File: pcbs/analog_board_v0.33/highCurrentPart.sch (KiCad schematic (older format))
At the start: 23 parts, among them J6 CONN_01X02, J7 CONN_01X02, J8 CONN_01X02, J9 CONN_01X02, Q1 MMBT3904, U3 LM358, U4 ICL7660S, U5 ICL7660S

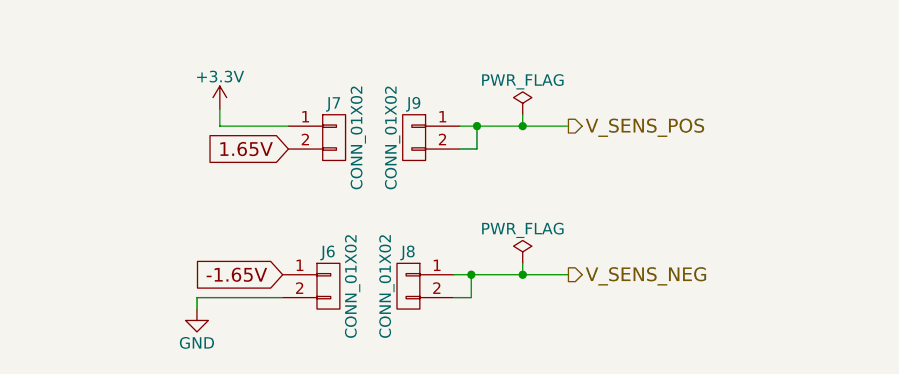
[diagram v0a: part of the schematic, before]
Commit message: Finished new BOM.
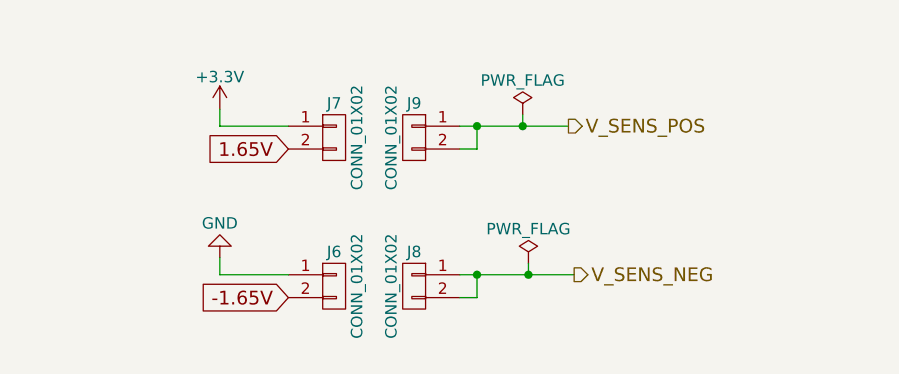
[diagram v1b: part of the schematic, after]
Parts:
- R10: Farnell 1632456 -> 9237364
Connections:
- net -1.65V: now also J6.2 (P2); no longer J6.1 (P1)
- net GND: now also J6.1 (P1); no longer J6.2 (P2)
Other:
- moved on the sheet: J6, J8
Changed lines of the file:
@@
 F 2 "Resistors_SMD:R_0805" V 1055 4025 50  0001 C CNN
 F 3 "" H 1125 4025 50  0000 C CNN
-F 4 "1632456" V 1125 4025 60  0001 C CNN "Farnell"
+F 4 "9237364" V 1125 4025 60  0001 C CNN "Farnell"
 	1    1125 4025
 	1    0    0    -1
@@
 	1    0    0    -1
 $EndComp
-Wire Wire Line
-	3575 5950 3875 5950
-Wire Wire Line
-	3575 5875 3575 5950
 Text HLabel 5100 5950 2    60   Output ~ 0
 V_SENS_POS
@@
 L CONN_01X02 J6
 U 1 1 5993FBA5
-P 4050 6650
-F 0 "J6" H 4050 6800 50  0000 C CNN
-F 1 "CONN_01X02" V 4150 6650 50  0000 C CNN
-F 2 "Samtec Connectors:Samtec-PHT-1-2-01-L-S" H 4050 6650 50  0001 C CNN
-F 3 "" H 4050 6650 50  0001 C CNN
-	1    4050 6650
+P 4075 6650
+F 0 "J6" H 4075 6800 50  0000 C CNN
+F 1 "CONN_01X02" V 4175 6650 50  0000 C CNN
+F 2 "Samtec Connectors:Samtec-PHT-1-2-01-L-S" H 4075 6650 50  0001 C CNN
+F 3 "" H 4075 6650 50  0001 C CNN
+	1    4075 6650
 	1    0    0    -1
 $EndComp
@@
 L CONN_01X02 J8
 U 1 1 5993FBAB
-P 4400 6650
-F 0 "J8" H 4400 6800 50  0000 C CNN
-F 1 "CONN_01X02" V 4500 6650 50  0000 C CNN
-F 2 "Samtec Connectors:Samtec-PHT-1-2-01-L-S" H 4400 6650 50  0001 C CNN
-F 3 "" H 4400 6650 50  0001 C CNN
-	1    4400 6650
+P 4425 6650
+F 0 "J8" H 4425 6800 50  0000 C CNN
+F 1 "CONN_01X02" V 4525 6650 50  0000 C CNN
+F 2 "Samtec Connectors:Samtec-PHT-1-2-01-L-S" H 4425 6650 50  0001 C CNN
+F 3 "" H 4425 6650 50  0001 C CNN
+	1    4425 6650
 	-1   0    0    -1
 $EndComp
-Text HLabel 5100 6600 2    60   Output ~ 0
+Text HLabel 5125 6600 2    60   Output ~ 0
 V_SENS_NEG
 Wire Wire Line
-	4600 6600 5100 6600
-Wire Wire Line
-	4600 6700 4675 6700
-Wire Wire Line
-	4675 6700 4675 6600
-Connection ~ 4675 6600
-Text GLabel 3850 6600 0    60   Input ~ 0
+	4625 6600 5125 6600
+Wire Wire Line
+	4625 6700 4700 6700
+Wire Wire Line
+	4700 6700 4700 6600
+Connection ~ 4700 6600
+Text GLabel 3875 6700 0    60   Input ~ 0
 -1.65V
 $Comp
 L GND #PWR039
 U 1 1 5993FFC9
-P 3475 6750
-F 0 "#PWR039" H 3475 6500 50  0001 C CNN
-F 1 "GND" H 3475 6600 50  0000 C CNN
-F 2 "" H 3475 6750 50  0001 C CNN
-F 3 "" H 3475 6750 50  0001 C CNN
-	1    3475 6750
-	1    0    0    -1
-$EndComp
-Wire Wire Line
-	3475 6750 3475 6700
-Wire Wire Line
-	3475 6700 3850 6700
+P 3575 6525
+F 0 "#PWR039" H 3575 6275 50  0001 C CNN
+F 1 "GND" H 3575 6375 50  0000 C CNN
+F 2 "" H 3575 6525 50  0001 C CNN
+F 3 "" H 3575 6525 50  0001 C CNN
+	1    3575 6525
+	-1   0    0    1
+$EndComp
 Wire Wire Line
 	6750 2325 7825 2325
@@
 L PWR_FLAG #FLG041
 U 1 1 599AF782
-P 4900 6550
-F 0 "#FLG041" H 4900 6625 50  0001 C CNN
-F 1 "PWR_FLAG" H 4900 6700 50  0000 C CNN
-F 2 "" H 4900 6550 50  0001 C CNN
-F 3 "" H 4900 6550 50  0001 C CNN
-	1    4900 6550
+P 4925 6550
+F 0 "#FLG041" H 4925 6625 50  0001 C CNN
+F 1 "PWR_FLAG" H 4925 6700 50  0000 C CNN
+F 2 "" H 4925 6550 50  0001 C CNN
+F 3 "" H 4925 6550 50  0001 C CNN
+	1    4925 6550
 	1    0    0    -1
 $EndComp
@@
 Connection ~ 4900 5950
 Wire Wire Line
-	4900 6550 4900 6600
-Connection ~ 4900 6600
+	4925 6550 4925 6600
+Connection ~ 4925 6600
 $Comp
 L PWR_FLAG #FLG043
@@
 	10325 1475 10325 1625
 Connection ~ 10325 1625
+Wire Wire Line
+	3575 6525 3575 6600
+Wire Wire Line
+	3575 6600 3875 6600
+Wire Wire Line
+	3575 5875 3575 5950
+Wire Wire Line
+	3575 5950 3875 5950
 $EndSCHEMATC
